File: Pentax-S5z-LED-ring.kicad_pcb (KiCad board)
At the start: 2 copper layers, 40 x 40 mm, 32 parts

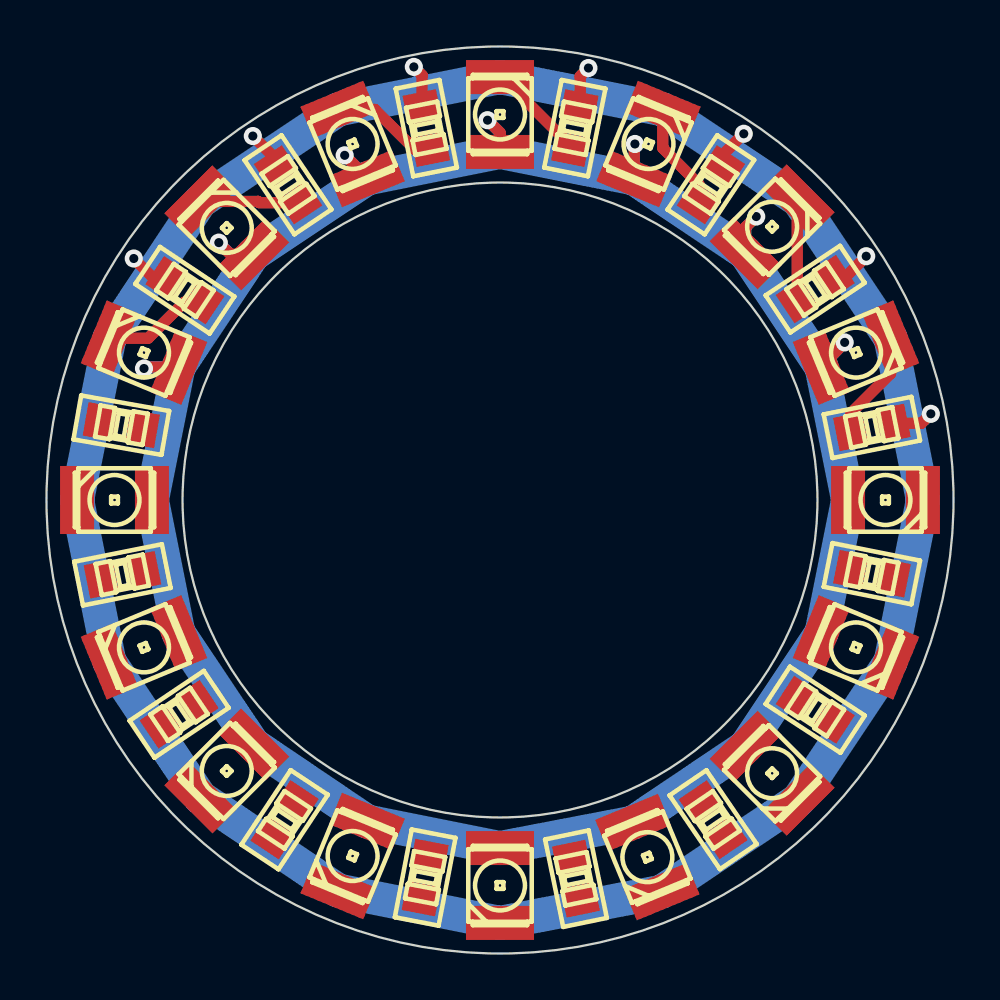
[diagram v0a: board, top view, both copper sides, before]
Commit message: Tweaks.
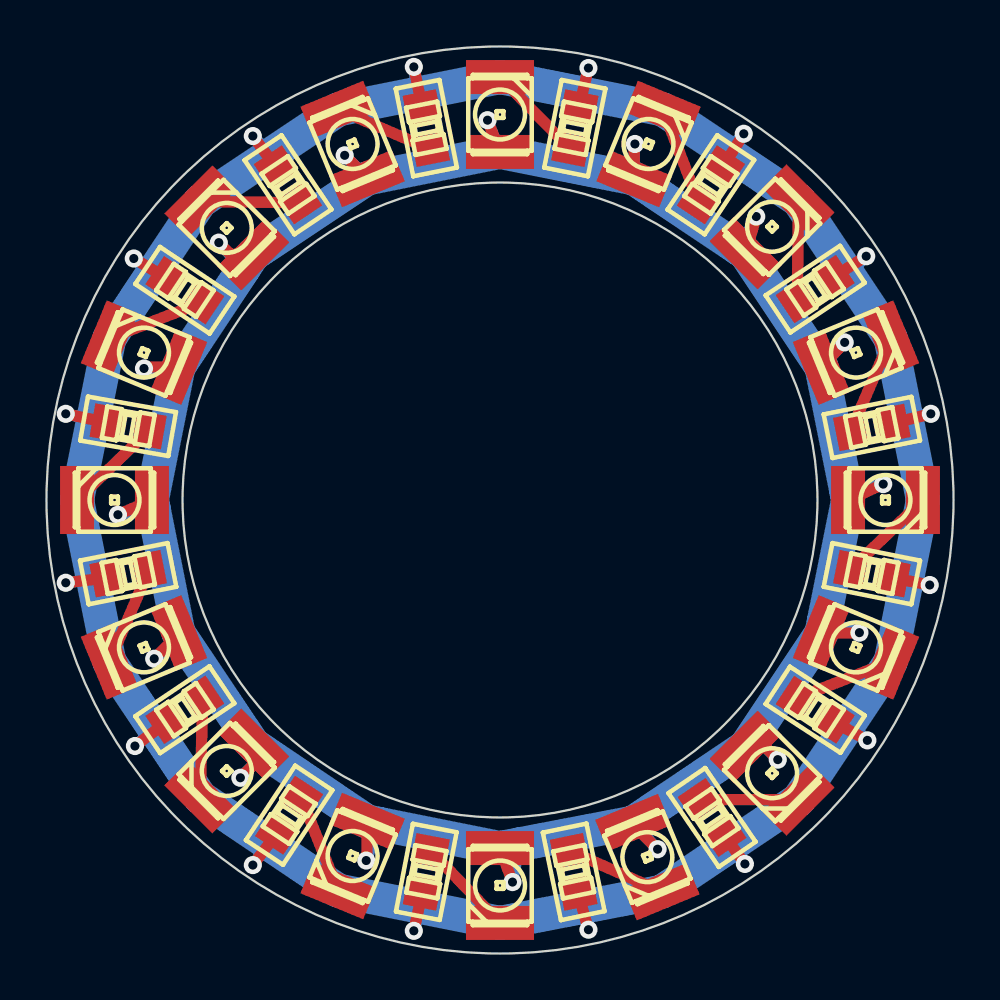
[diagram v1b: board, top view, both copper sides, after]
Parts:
- moved R11 0.32 mm to (51.1, 74.2), turned to 213.9 degrees
- moved R8 0.32 mm to (68.2, 81.4), turned to 281.7 degrees
- moved R13 0.30 mm to (48.6, 61.8)
- moved R10 0.28 mm to (55.7, 78.9), turned to 236.5 degrees
- moved R12 0.25 mm to (48.6, 68.2), turned to 191.3 degrees
- moved R9 0.25 mm to (61.8, 81.4), turned to 259.1 degrees
- moved R7 0.11 mm to (74.3, 79.0), turned to 304.3 degrees
- turned R6 to 326.9 degrees
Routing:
- net N-0000018: track 118.2 -> 148.4 mm, vias 7 -> 16
- net N-0000017: track 137.3 -> 163.4 mm, vias 7 -> 16
- net N-000009: track 0.00 -> 4.71 mm
- net N-000008: track 0.00 -> 4.46 mm
- net N-0000013: track 0.00 -> 4.43 mm
- net N-0000010: track 0.00 -> 4.43 mm
- net N-0000012: track 0.00 -> 4.43 mm
- net N-000006: track 0.00 -> 4.42 mm
- net N-000005: track 0.00 -> 4.42 mm
- net N-0000011: track 0.00 -> 4.40 mm
- net N-000007: track 0.00 -> 4.35 mm
